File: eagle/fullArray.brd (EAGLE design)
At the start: 69 parts

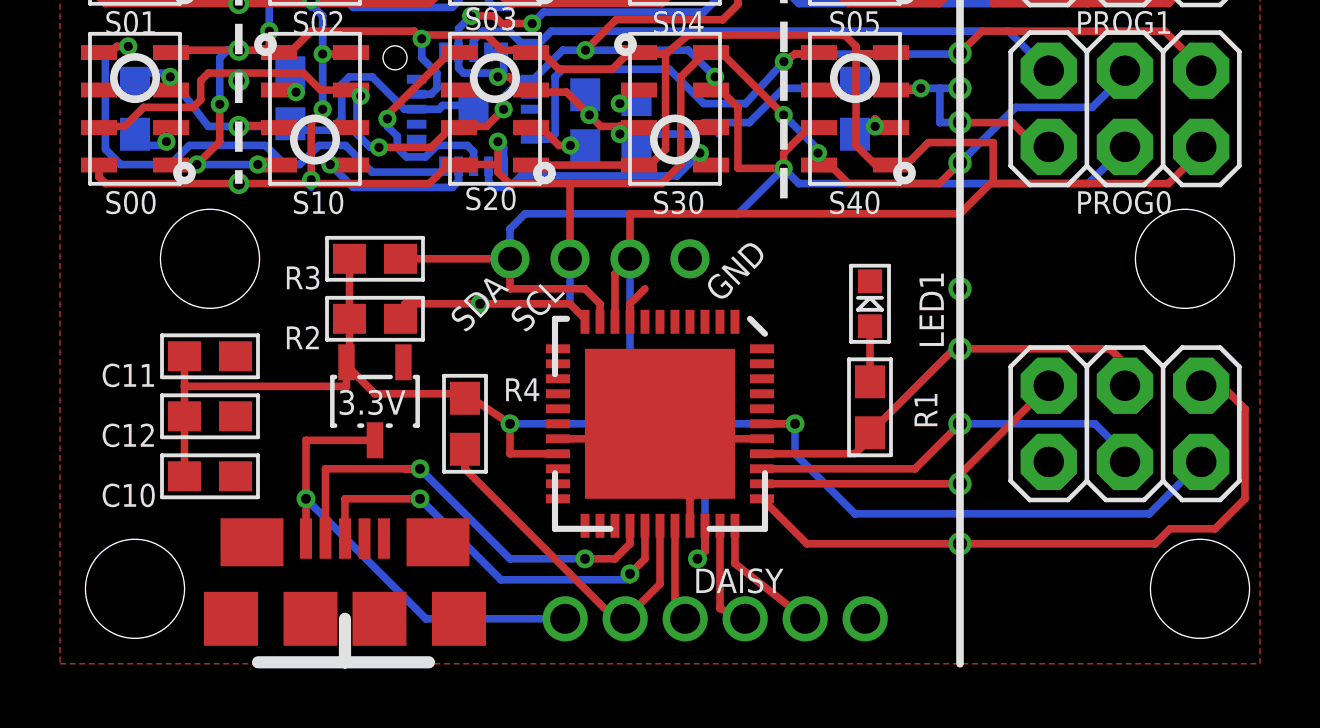
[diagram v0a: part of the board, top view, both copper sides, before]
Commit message: square up mounting holes
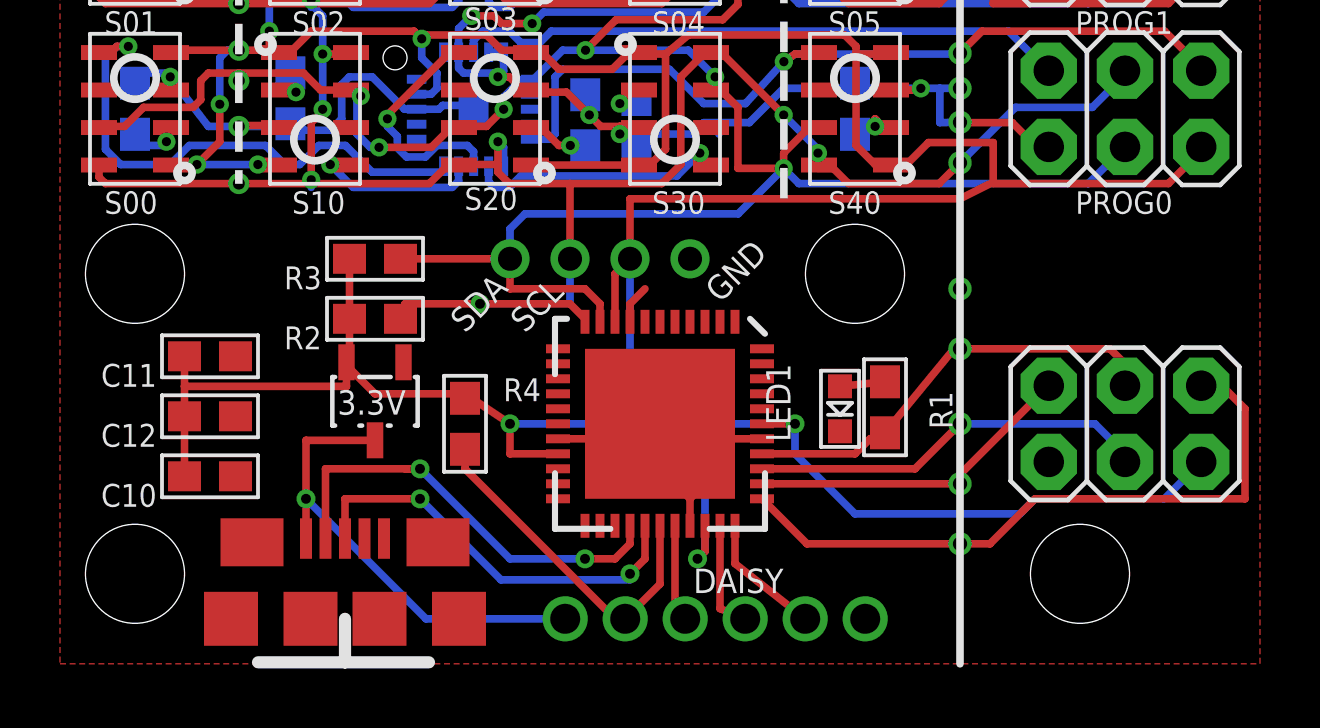
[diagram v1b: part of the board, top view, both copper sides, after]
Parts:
- moved U$4 11.0 mm to (6.50, 13.0)
- moved U$2 4.03 mm to (14.0, 3.00)
- moved LED1 3.64 mm to (6.00, 8.50), turned to 180 degrees
- moved U$3 2.55 mm to (-17.5, 13.0)
- moved R1 0.50 mm to (7.50, 8.55)
- moved U$1 0.50 mm to (-17.5, 3.00)
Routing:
- net PDI-DATA: vias 0 -> 1
- net PDI-CLK: vias 0 -> 1
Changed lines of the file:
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@@
 <attribute name="VALUE" x="19.31" y="12.445" size="1.27" layer="27" rot="R180"/>
 </element>
-<element name="R1" library="nonolith" package="0603" value="" x="7" y="8.55" smashed="yes" rot="R90">
-<attribute name="NAME" x="9.246" y="7.828" size="0.762" layer="25" font="vector" ratio="10" rot="R90"/>
-</element>
-<element name="LED1" library="microbuilder" package="CHIPLED_0603" value="" x="7" y="12" smashed="yes">
-<attribute name="NAME" x="8.65" y="13.1" size="0.8128" layer="25" font="vector" ratio="12" rot="R270"/>
-<attribute name="VALUE" x="8.143" y="10.73" size="0.4064" layer="27" rot="R90"/>
+<element name="R1" library="nonolith" package="0603" value="" x="7.5" y="8.55" smashed="yes" rot="R90">
+<attribute name="NAME" x="9.746" y="7.828" size="0.762" layer="25" font="vector" ratio="10" rot="R90"/>
+</element>
+<element name="LED1" library="microbuilder" package="CHIPLED_0603" value="" x="6" y="8.5" smashed="yes" rot="R180">
+<attribute name="NAME" x="4.35" y="7.4" size="0.8128" layer="25" font="vector" ratio="12" rot="R90"/>
+<attribute name="VALUE" x="4.857" y="9.77" size="0.4064" layer="27" rot="R270"/>
 </element>
 <element name="R2" library="nonolith" package="0603" value="" x="-9.5" y="11.5" rot="R180"/>
 <element name="R3" library="nonolith" package="0603" value="" x="-9.5" y="13.5" rot="R180"/>
-<element name="U$1" library="nonolith" package="STAND-OFF" value="" x="-17.5" y="2.5"/>
-<element name="U$2" library="nonolith" package="STAND-OFF" value="" x="18" y="2.5"/>
+<element name="U$1" library="nonolith" package="STAND-OFF" value="" x="-17.5" y="3"/>
+<element name="U$2" library="nonolith" package="STAND-OFF" value="" x="14" y="3"/>
 <element name="DAISY" library="nonolith" package="1X06_ROUND_2MM" value="" x="7" y="1.5" smashed="yes" rot="R180">
 <attribute name="NAME" x="4.1162" y="3.1712" size="0.8128" layer="25" font="vector" ratio="12" rot="R180"/>
@@
 <attribute name="VALUE" x="-6.27" y="10.325" size="1.27" layer="27"/>
 </element>
-<element name="U$3" library="nonolith" package="STAND-OFF" value="" x="-15" y="13.5" smashed="yes"/>
-<element name="U$4" library="nonolith" package="STAND-OFF" value="" x="17.5" y="13.5"/>
+<element name="U$3" library="nonolith" package="STAND-OFF" value="" x="-17.5" y="13" smashed="yes"/>
+<element name="U$4" library="nonolith" package="STAND-OFF" value="" x="6.5" y="13"/>
 <element name="JP1" library="nonolith" package="1X01_2MM" value="" x="1" y="13.5" smashed="yes">
 <attribute name="VALUE" x="-0.27" y="10.325" size="1.27" layer="27"/>
@@
 <wire x1="-15.85" y1="9.25" x2="-10.45" y2="9.25" width="0.254" layer="1"/>
 <wire x1="-10.45" y1="9.25" x2="-10.45" y2="10.05" width="0.254" layer="1"/>
-<wire x1="18.04" y1="6.73" x2="16.31" y2="5" width="0.254" layer="16"/>
-<wire x1="16.31" y1="5" x2="6.5" y2="5" width="0.254" layer="16"/>
+<wire x1="18.04" y1="6.73" x2="16.81" y2="5.5" width="0.254" layer="16"/>
+<wire x1="16.81" y1="5.5" x2="12.5" y2="5.5" width="0.254" layer="16"/>
+<wire x1="12.5" y1="5.5" x2="12" y2="5" width="0.254" layer="16"/>
+<wire x1="12" y1="5" x2="6.5" y2="5" width="0.254" layer="16"/>
 <wire x1="6.5" y1="5" x2="4.5" y2="7" width="0.254" layer="16"/>
 <wire x1="4.5" y1="7" x2="4.5" y2="8" width="0.254" layer="16"/>
-<wire x1="-1" y1="13.5" x2="-1" y2="15" width="0.254" layer="1"/>
-<wire x1="-1" y1="15" x2="10" y2="15" width="0.254" layer="1"/>
-<wire x1="10" y1="15" x2="11" y2="16" width="0.254" layer="1"/>
+<wire x1="-1" y1="13.5" x2="-1" y2="15.5" width="0.254" layer="1"/>
+<wire x1="-1" y1="15.5" x2="10" y2="15.5" width="0.254" layer="1"/>
+<wire x1="10" y1="15.5" x2="11" y2="16" width="0.254" layer="1"/>
 <wire x1="11.107" y1="16.008" x2="11" y2="16" width="0" layer="19" extent="1-1"/>
 </signal>
@@
 <wire x1="15" y1="10.5" x2="15.5" y2="10" width="0.254" layer="1"/>
 <wire x1="15.5" y1="10" x2="15.5" y2="9.27" width="0.254" layer="1"/>
-<wire x1="7" y1="7.7" x2="9.8" y2="10.5" width="0.254" layer="1"/>
+<wire x1="7.5" y1="7.7" x2="9.8" y2="10.5" width="0.254" layer="1"/>
 <via x="10" y="10.5" extent="1-16" drill="0.475" shape="octagon"/>
 <wire x1="6.5" y1="7" x2="7" y2="7.5" width="0.254" layer="1"/>
-<wire x1="7" y1="7.7" x2="7" y2="7.5" width="0.254" layer="1"/>
+<wire x1="7.5" y1="7.7" x2="7" y2="7.5" width="0.254" layer="1"/>
 </signal>
 <signal name="PR1-P">
 <contactref element="R1" pad="2"/>
 <contactref element="LED1" pad="A"/>
-<wire x1="7" y1="11.25" x2="7" y2="9.4" width="0.254" layer="1"/>
+<wire x1="6" y1="9.25" x2="7.5" y2="9.4" width="0.254" layer="1"/>
 </signal>
 <signal name="BOOTLOAD">
@@
 <wire x1="18.73" y1="9.27" x2="18.04" y2="9.27" width="0.254" layer="1"/>
 <wire x1="3.4" y1="5.5" x2="4.9" y2="4" width="0.254" layer="1"/>
-<wire x1="4.9" y1="4" x2="16.5" y2="4" width="0.254" layer="1"/>
-<wire x1="16.5" y1="4" x2="17" y2="4.5" width="0.254" layer="1"/>
-<wire x1="17" y1="4.5" x2="18.5" y2="4.5" width="0.254" layer="1"/>
-<wire x1="18.5" y1="4.5" x2="19.5" y2="5.5" width="0.254" layer="1"/>
+<wire x1="4.9" y1="4" x2="10" y2="4" width="0.254" layer="1"/>
+<wire x1="10" y1="4" x2="11" y2="4" width="0.254" layer="1"/>
+<wire x1="11" y1="4" x2="12.5" y2="5.5" width="0.254" layer="1"/>
+<wire x1="12.5" y1="5.5" x2="19.5" y2="5.5" width="0.254" layer="1"/>
+<via x="10" y="4" extent="1-16" drill="0.475" shape="octagon"/>
 </signal>
 <signal name="PDI-CLK">
@@
 <wire x1="12.96" y1="9.27" x2="9.69" y2="6" width="0.254" layer="1"/>
 <wire x1="9.69" y1="6" x2="3.4" y2="6" width="0.254" layer="1"/>
+<via x="10" y="6" extent="1-16" drill="0.475" shape="octagon"/>
+<wire x1="9.69" y1="6" x2="10" y2="6" width="0" layer="19" extent="1-1"/>
 </signal>
 <signal name="5V">
@@
 <contactref element="UC3" pad="11"/>
 </signal>
-<signal name="N$1">
-<via x="10" y="6" extent="1-16" drill="0.475" shape="octagon"/>
-</signal>
-<signal name="N$2">
-<via x="10" y="4" extent="1-16" drill="0.475" shape="octagon"/>
-</signal>
 <signal name="N$3">

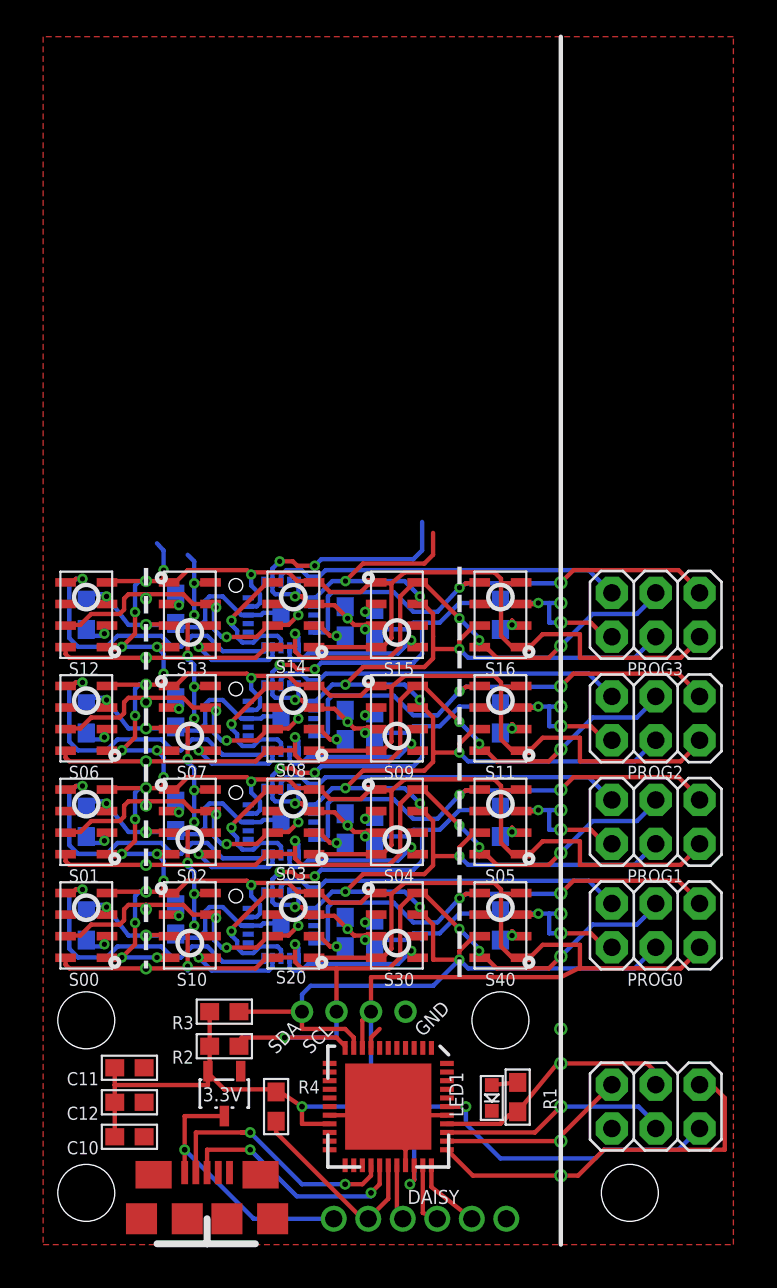
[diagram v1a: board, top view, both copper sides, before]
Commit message: full 8 rows with standardized naming
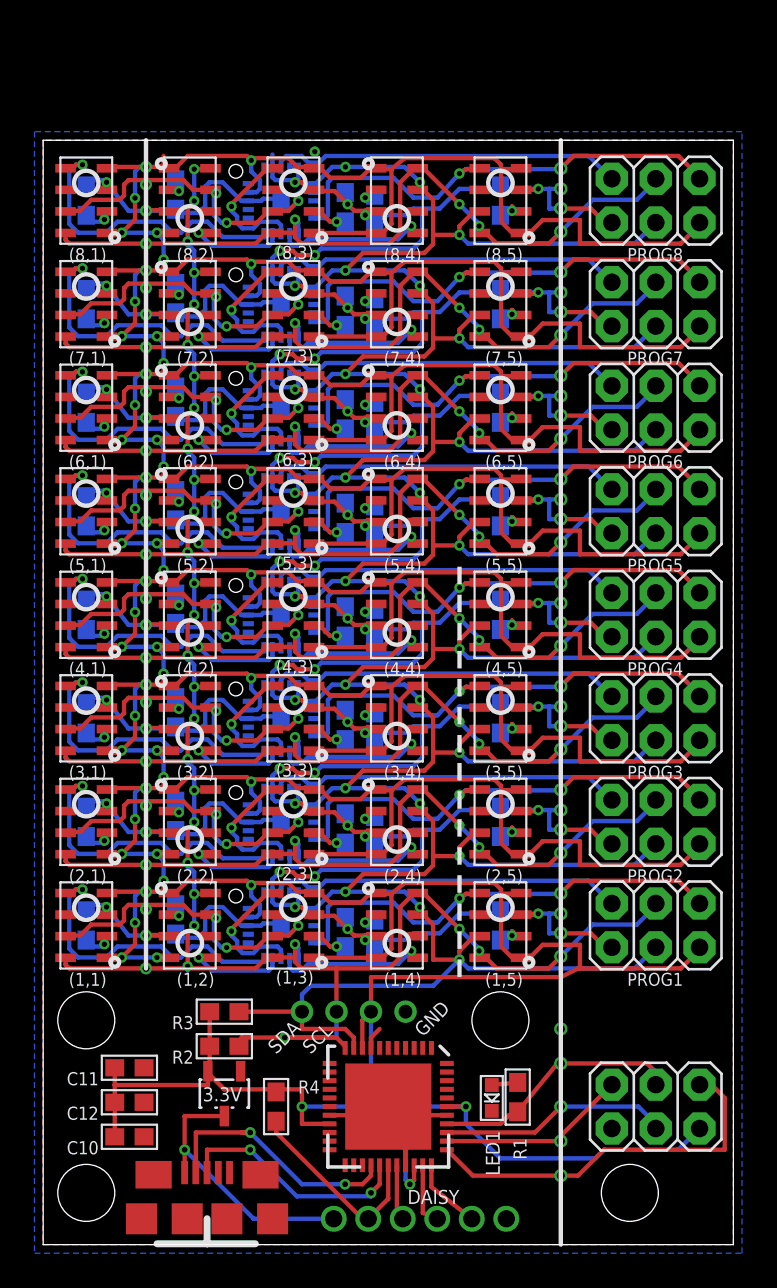
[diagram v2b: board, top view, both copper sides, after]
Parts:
- removed PROG0: (no value), nonolith:2X03
- added (5,1), (5,2), (5,3), (5,4), (5,5), (6,1), (6,2), (6,3), (6,4), (6,5), (7,1), (7,2), (7,3), (7,4), (7,5), (8,1), (8,2), (8,3), (8,4), (8,5): MPL115A, nonolith:LGA-8
- added AT5, AT6, AT7, AT8: ATTINY24QFN, nonolith:QFN20
- added C23, C24, C25, C26, C27, C28, C29, C30, C31, C32, C33, C34, C35, C36, C37, C38, C39, C40, C41, C42: (no value), nonolith:0603
- added PROG4, PROG5, PROG6, PROG7, PROG8: (no value), nonolith:2X03
- moved PROG1 6.00 mm to (15.5, 18.5)
- moved PROG2 6.00 mm to (15.5, 24.5)
- moved PROG3 6.00 mm to (15.5, 30.5)
- renumbered S00 to (1,1), S01 to (2,1), S02 to (2,2), S03 to (2,3), S04 to (2,4), S05 to (2,5), S06 to (3,1), S07 to (3,2), S08 to (3,3), S09 to (3,4), S10 to (1,2), S11 to (3,5), S12 to (4,1), S13 to (4,2), S14 to (4,3), S15 to (4,4), S16 to (4,5), S20 to (1,3), S30 to (1,4), S40 to (1,5), UC0 to AT1, UC1 to AT2, UC2 to AT3, UC3 to AT4
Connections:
- net RST03 renamed RST14
- removed net RST00: (1,1).5, AT1.5
- removed net RST01: (2,1).5, AT2.5
- removed net RST02: (3,1).5, AT3.5
- removed net RST10: (1,2).5, AT1.4
- removed net RST20: (1,3).5, AT1.3
- removed net RST30: (1,4).5, AT1.2
- removed net RST40: (1,5).5, AT1.20, PROG0.1
- new net ADDR04: AT5.11
- new net ADDR05: AT6.11
- new net ADDR06: AT7.11
- new net ADDR07: AT8.11
- new net CAP17: (5,3).2, C25.1
- new net CAP18: (5,4).2, C26.1
- new net CAP19: (5,5).2, C27.1
- new net CAP21: (5,1).2, C23.1
- new net CAP22: (5,2).2, C24.1
- new net CAP23: (6,3).2, C30.1
- new net CAP24: (6,4).2, C31.1
- new net CAP25: (6,5).2, C32.1
- new net CAP26: (6,1).2, C28.1
- new net CAP27: (6,2).2, C29.1
- new net CAP28: (7,3).2, C35.1
- new net CAP29: (7,4).2, C36.1
- new net CAP31: (7,5).2, C37.1
- new net CAP32: (7,1).2, C33.1
- new net CAP33: (7,2).2, C34.1
- new net CAP34: (8,3).2, C40.1
- new net CAP35: (8,4).2, C41.1
- new net CAP36: (8,5).2, C42.1
- new net CAP37: (8,1).2, C38.1
- new net CAP38: (8,2).2, C39.1
- new net RESET4: AT4.13, PROG4.5
- new net RESET5: AT5.13, PROG5.5
- new net RESET6: AT6.13, PROG6.5
- new net RESET7: AT7.13, PROG7.5
- new net RESET8: AT8.13, PROG8.5
- new net RST15: (5,1).5, AT5.5
- new net RST16: (6,1).5, AT6.5
- new net RST17: (7,1).5, AT7.5
- new net RST18: (8,1).5, AT8.5
- new net RST24: (4,2).5, AT4.4
- new net RST25: (5,2).5, AT5.4
- new net RST26: (6,2).5, AT6.4
- new net RST27: (7,2).5, AT7.4
- new net RST28: (8,2).5, AT8.4
- new net RST34: (4,3).5, AT4.3
- new net RST35: (5,3).5, AT5.3
- new net RST36: (6,3).5, AT6.3
- new net RST37: (7,3).5, AT7.3
- new net RST38: (8,3).5, AT8.3
- new net RST44: (4,4).5, AT4.2
- new net RST45: (5,4).5, AT5.2
- new net RST46: (6,4).5, AT6.2
- new net RST47: (7,4).5, AT7.2
- new net RST48: (8,4).5, AT8.2
- new net RST51: (1,5).5, AT1.20, PROG1.1
- new net RST52: (2,5).5, AT2.20, PROG2.1
- new net RST53: (3,5).5, AT3.20, PROG3.1
- new net RST54: (4,5).5, AT4.20, PROG4.1
- new net RST55: (5,5).5, AT5.20, PROG5.1
- new net RST56: (6,5).5, AT6.20, PROG6.1
- new net RST57: (7,5).5, AT7.20, PROG7.1
- new net RST58: (8,5).5, AT8.20, PROG8.1
- net 3.3V: now also (5,1).1, (5,1).4, (5,2).1, (5,2).4, (5,3).1, (5,3).4, (5,4).1, (5,4).4, (5,5).1, (5,5).4, (6,1).1, (6,1).4, (6,2).1, (6,2).4, (6,3).1, (6,3).4, (6,4).1, (6,4).4, (6,5).1, (6,5).4, (7,1).1, (7,1).4, (7,2).1, (7,2).4, (7,3).1, (7,3).4, (7,4).1, (7,4).4, (7,5).1, (7,5).4, (8,1).1, (8,1).4, (8,2).1, (8,2).4, (8,3).1, (8,3).4, (8,4).1, (8,4).4, (8,5).1, (8,5).4, AT5.9, AT6.9, AT7.9, AT8.9, PROG4.2, PROG5.2, PROG6.2, PROG7.2, PROG8.2; no longer PROG0.2
- net GND: now also (5,1).3, (5,2).3, (5,3).3, (5,4).3, (5,5).3, (6,1).3, (6,2).3, (6,3).3, (6,4).3, (6,5).3, (7,1).3, (7,2).3, (7,3).3, (7,4).3, (7,5).3, (8,1).3, (8,2).3, (8,3).3, (8,4).3, (8,5).3, AT5.0, AT5.12, AT5.14, AT5.15, AT5.8, AT6.0, AT6.12, AT6.14, AT6.15, AT6.8, AT7.0, AT7.12, AT7.14, AT7.15, AT7.8, AT8.0, AT8.12, AT8.14, AT8.15, AT8.8, C23.2, C24.2, C25.2, C26.2, C27.2, C28.2, C29.2, C30.2, C31.2, C32.2, C33.2, C34.2, C35.2, C36.2, C37.2, C38.2, C39.2, C40.2, C41.2, C42.2, PROG4.6, PROG5.6, PROG6.6, PROG7.6, PROG8.6; no longer PROG0.6
- net RESET0: no longer PROG0.5
- net RESET1: no longer AT2.13
- net RESET2: now also AT2.13; no longer AT3.13
- net RESET3: now also AT3.13; no longer AT4.13
- net RST11: now also (1,1).5, AT1.5; no longer (2,2).5, AT2.4
- net RST12: now also (2,1).5, AT2.5; no longer (3,2).5, AT3.4
- net RST13: now also (3,1).5, AT3.5; no longer (4,2).5, AT4.4
- net RST21: now also (1,2).5, AT1.4; no longer (2,3).5, AT2.3
- net RST22: now also (2,2).5, AT2.4; no longer (3,3).5, AT3.3
- net RST23: now also (3,2).5, AT3.4; no longer (4,3).5, AT4.3
- net RST31: now also (1,3).5, AT1.3; no longer (2,4).5, AT2.2
- net RST32: now also (2,3).5, AT2.3; no longer (3,4).5, AT3.2
- net RST33: now also (3,3).5, AT3.3; no longer (4,4).5, AT4.2
- net RST41: now also (1,4).5, AT1.2; no longer (2,5).5, AT2.20, PROG1.1
- net RST42: now also (2,4).5, AT2.2; no longer (3,5).5, AT3.20, PROG2.1
- net RST43: now also (3,4).5, AT3.2; no longer (4,5).5, AT4.20, PROG3.1
- net SCL: now also (5,1).8, (5,2).8, (5,3).8, (5,4).8, (5,5).8, (6,1).8, (6,2).8, (6,3).8, (6,4).8, (6,5).8, (7,1).8, (7,2).8, (7,3).8, (7,4).8, (7,5).8, (8,1).8, (8,2).8, (8,3).8, (8,4).8, (8,5).8, AT5.1, AT6.1, AT7.1, AT8.1, PROG4.3, PROG5.3, PROG6.3, PROG7.3, PROG8.3; no longer PROG0.3
- net SDA: now also (5,1).7, (5,2).7, (5,3).7, (5,4).7, (5,5).7, (6,1).7, (6,2).7, (6,3).7, (6,4).7, (6,5).7, (7,1).7, (7,2).7, (7,3).7, (7,4).7, (7,5).7, (8,1).7, (8,2).7, (8,3).7, (8,4).7, (8,5).7, AT5.16, AT6.16, AT7.16, AT8.16, PROG4.4, PROG5.4, PROG6.4, PROG7.4, PROG8.4; no longer PROG0.4
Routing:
- net 3.3V: track 340.6 -> 603.2 mm, vias 27 -> 50
- net GND: track 262.7 -> 503.1 mm, vias 40 -> 80
- net SCL: track 228.8 -> 441.8 mm, vias 33 -> 65
- net SDA: track 229.7 -> 432.2 mm, vias 28 -> 56
- net RST58: track 0.00 -> 27.8 mm, vias 0 -> 2
- net RST57: track 0.00 -> 27.8 mm, vias 0 -> 2
- net RST40: track 27.8 -> 0.00 mm, vias 2 -> 0
- net RST56: track 0.00 -> 27.8 mm, vias 0 -> 2
- net RST53: track 0.00 -> 27.8 mm, vias 0 -> 2
- net RST52: track 0.00 -> 27.8 mm, vias 0 -> 2
- net RST51: track 0.00 -> 27.8 mm, vias 0 -> 2
- net RST55: track 0.00 -> 27.1 mm, vias 0 -> 2
- net RST54: track 0.00 -> 27.1 mm, vias 0 -> 2
- net RESET1: track 20.6 -> 0.00 mm
- net RESET8: track 0.00 -> 20.6 mm
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- added copper zone on layer 16, net GND
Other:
- board outline added: 40 x 64 mm
